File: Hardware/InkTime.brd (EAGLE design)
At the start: 36 x 36 mm, 50 parts, among them IC1 BQ25180YBGR, IC2 DRV2605YZFR, IC3 BMA423, IC9 RT6160AWSC, J1 EPD_24P, J2 TC2030, J4 USB-C, U1 nRF52840, U3 MAX17048G+T10, X1 32MHz, X2 32.768kHz

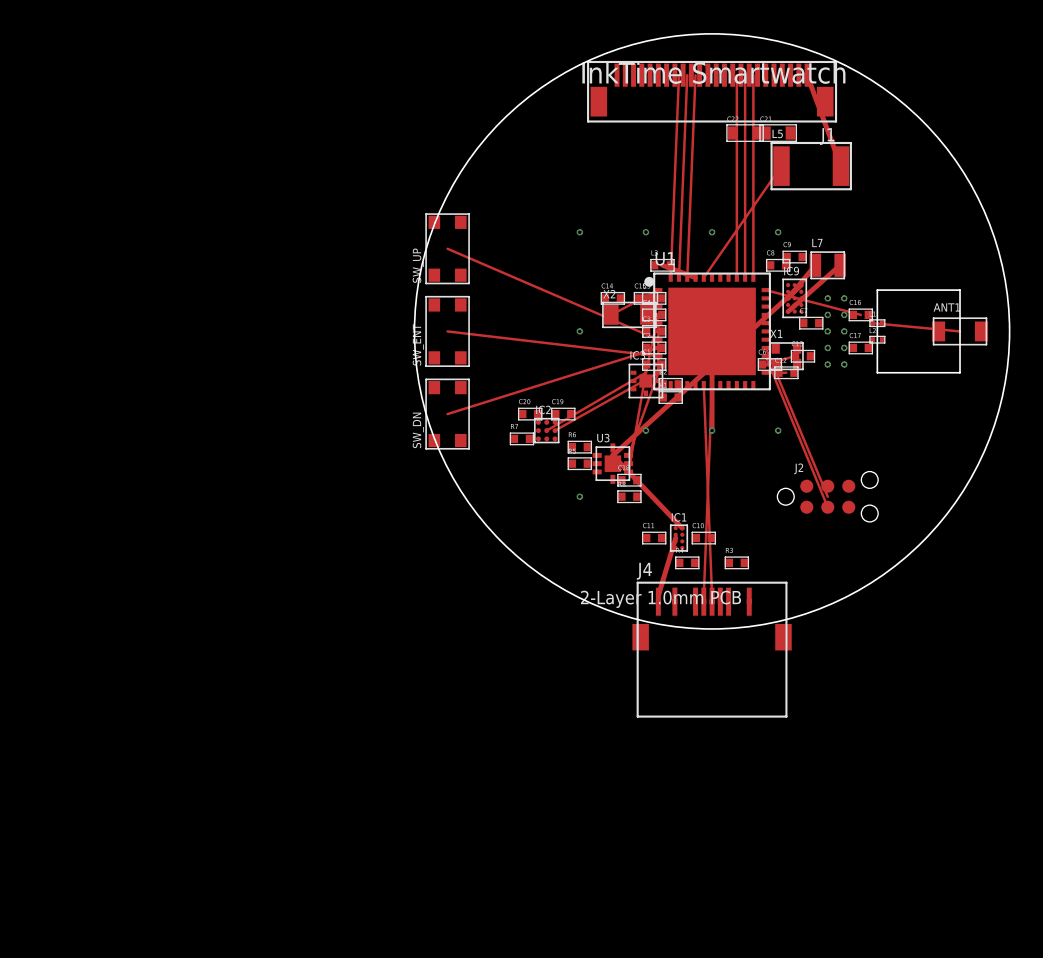
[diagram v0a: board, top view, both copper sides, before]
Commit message: Update 1
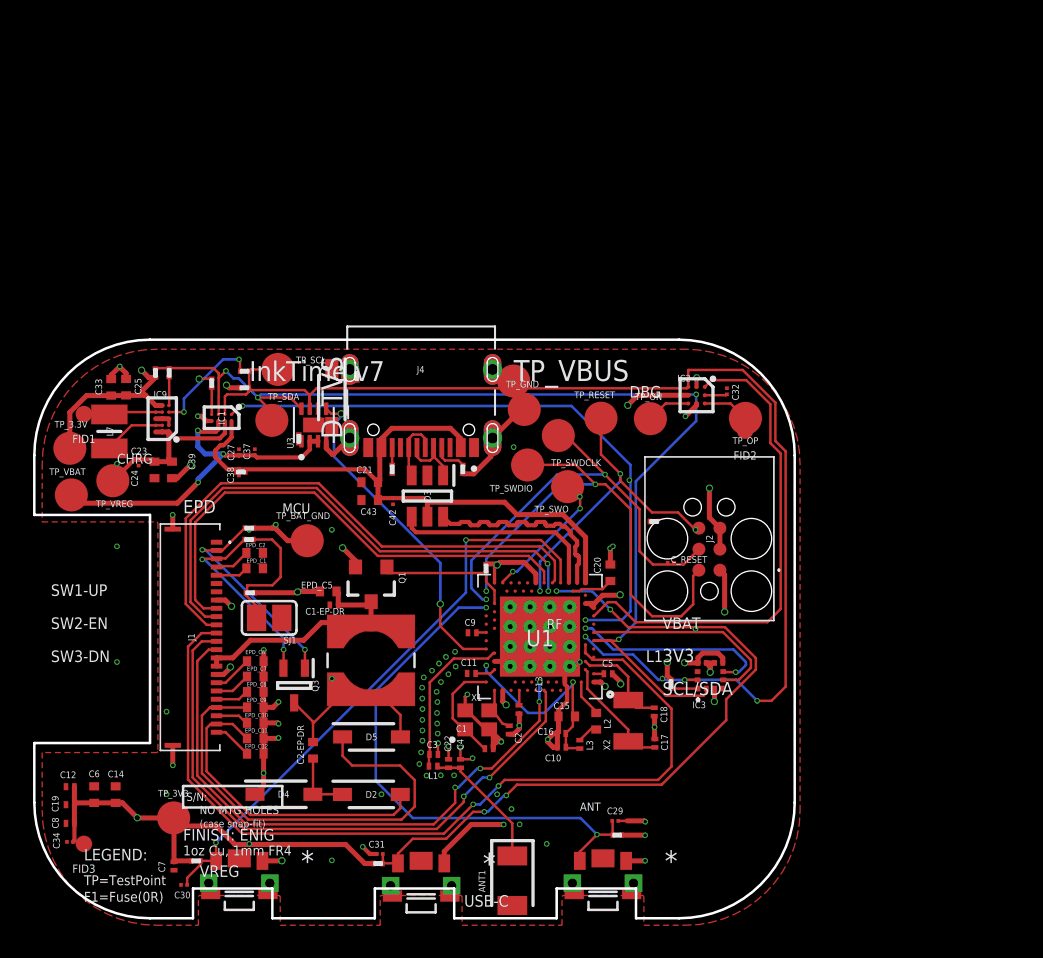
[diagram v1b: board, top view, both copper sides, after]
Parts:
- removed R1: 10k, InkTime_v5:GENERIC_0402
- removed R6: 100k, InkTime_v5:GENERIC_0402
- added C1-EP-DR, C24, C39: 10uF, InkTime_v5:NORDIC_NRF_3_RESC0402_L
- added C2-EP-DR: 4.7uF/25V, InkTime_v5:NORDIC_NRF_3_RESC0402_L
- added C23, C27, C34, C42: 0.1uF, InkTime_v5:GRM011R60J152KE01L_2_CAPC0201X13N
- added C25, C33: 22uF, InkTime_v5:NORDIC_NRF_3_RESC0402_L
- added C29, C30, C31, C32, C37, C38: 1uF, InkTime_v5:GRM011R60J152KE01L_2_CAPC0201X13N
- added C43: 4.7uF, InkTime_v5:NORDIC_NRF_3_RESC0402_L
- added C_RESET: 100nF/10V, InkTime_v5:GRM011R60J152KE01L_2_CAPC0201X13N
- added D2, D4, D5: MBR0530, InkTime_v5:ESP32_C6_LIBRARY_5_SOD3716X135N
- added D3: USBLC6-2SC6Y, InkTime_v5:ESP32_C6_LIBRARY_3_SOT95P280X145-6N
- added D_TVS: MBR0530 (TVS), InkTime_v5:ESP32_C6_LIBRARY_5_SOD3716X135N
- added EPD_C1, EPD_C10, EPD_C11, EPD_C12, EPD_C2, EPD_C6, EPD_C7, EPD_C8, EPD_C9: 1uF/50V, InkTime_v5:NORDIC_NRF_3_RESC0402_L
- added EPD_C5: 0.1uF/50V, InkTime_v5:NORDIC_NRF_3_RESC0201_L
- added F1: 0R (FUSE), InkTime_v5:CPF0201D7K68C1_0201
- added Q1: 20V/4.2A/52mΩ/1.4W, InkTime_v5:ESP32_C6_LIBRARY_4_ESP32_C6_LIBRARY_4_ESP32_C6_LIBRARY_4_ESP32_C6_LIBRARY_4_ESP32_WROVER_SPARKFUN-DISCRETESE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
- added Q3: SI1308EDL-T1-GE3, InkTime_v5:ESP32_C6_LIBRARY_6_SOT65P210X110-3N
- added R17, R18: 3K3, InkTime_v5:CPF0201D7K68C1_0201
- added R1_EP_DR: 0.47, InkTime_v5:CPF0201D7K68C1_0201
- added R1_USB, R2_USB: 5K1, InkTime_v5:CPF0201D7K68C1_0201
- added R2_EP_DR, R9, R_PWR_EPD, R_RESET: 10K, InkTime_v5:CPF0201D7K68C1_0201
- added R_ALERT, R_PMIC_INT: 100K, InkTime_v5:CPF0201D7K68C1_0201
- added R_TYPE_SEL: 2.2, InkTime_v5:CPF0201D7K68C1_0201
- added SJ1: SJ, InkTime_v5:ESP32_C6_LIBRARY_7_JUMPER_SJ
- added TP_3.3V, TP_3V3, TP_BAT_GND, TP_GND, TP_ON, TP_OP, TP_RESET, TP_SCL, TP_SDA, TP_SWDCLK, TP_SWDIO, TP_SWO, TP_VBAT, TP_VREG: HECTOR_WATCH_1_TPTP20R, InkTime_v5:HECTOR_WATCH_1_TP20R
- added TP_VBUS: VBUS, InkTime_v5:HECTOR_WATCH_1_TP20R
- ANT1: value 2450AT18B100E -> 2450AT18B100E_2450AT18B100E
- C1, C2: value 100nF -> 12pF; device InkTime_v5:GENERIC_0402 -> InkTime_v5:NORDIC_NRF_3_RESC0201_L
- C10: value 1uF -> N.C.; device InkTime_v5:GENERIC_0402 -> InkTime_v5:NORDIC_NRF_3_RESC0201_L
- C11: value 4.7uF -> 100pF; device InkTime_v5:GENERIC_0402 -> InkTime_v5:NORDIC_NRF_3_RESC0201_L
- C12: value 12pF -> 100nF; device InkTime_v5:GENERIC_0402 -> InkTime_v5:NORDIC_NRF_3_RESC0201_L
- C13: value 12pF -> N.C.; device InkTime_v5:GENERIC_0402 -> InkTime_v5:NORDIC_NRF_3_RESC0201_L
- C14: value 6.8pF -> 4.7uF; device InkTime_v5:GENERIC_0402 -> InkTime_v5:NORDIC_NRF_3_RESC0402_L
- C15: value 6.8pF -> 1uF; device InkTime_v5:GENERIC_0402 -> InkTime_v5:NORDIC_NRF_3_RESC0402_L
- C16: value 0.8pF -> 47nF; device InkTime_v5:GENERIC_0402 -> InkTime_v5:NORDIC_NRF_3_RESC0201_L
- C17: value 0.5pF -> 12pF; device InkTime_v5:GENERIC_0402 -> InkTime_v5:NORDIC_NRF_3_RESC0201_L
- C18: value 1uF -> 12pF; device InkTime_v5:GENERIC_0402 -> InkTime_v5:NORDIC_NRF_3_RESC0201_L
- C19: value 1uF -> 100nF; device InkTime_v5:GENERIC_0402 -> InkTime_v5:NORDIC_NRF_3_RESC0201_L
- C20: value 100nF -> 4.7uF; device InkTime_v5:GENERIC_0402 -> InkTime_v5:NORDIC_NRF_3_RESC0402_L
- C21: device InkTime_v5:GENERIC_0603 -> InkTime_v5:NORDIC_NRF_3_RESC0402_L
- C22: value 1uF -> N.C.; device InkTime_v5:GENERIC_0603 -> InkTime_v5:NORDIC_NRF_3_RESC0201_L
- C3: value 100nF -> 1pF; device InkTime_v5:GENERIC_0402 -> InkTime_v5:NORDIC_NRF_3_RESC0201_L
- C4: value 1uF -> 1pF; device InkTime_v5:GENERIC_0402 -> InkTime_v5:NORDIC_NRF_3_RESC0201_L
- C5: device InkTime_v5:GENERIC_0402 -> InkTime_v5:NORDIC_NRF_3_RESC0201_L
- C6: device InkTime_v5:GENERIC_0402 -> InkTime_v5:NORDIC_NRF_3_RESC0402_L
- C7, C8: value 10uF -> 100nF; device InkTime_v5:GENERIC_0402 -> InkTime_v5:NORDIC_NRF_3_RESC0201_L
- C9: value 100nF -> 820pF (N.C.); device InkTime_v5:GENERIC_0402 -> InkTime_v5:NORDIC_NRF_3_RESC0201_L
- IC1: value BQ25180YBGR -> BQ25180YBGR_BQ25180YBGR
- IC2: value DRV2605YZFR -> DRV2605YZFR_DRV2605YZFR
- IC3: value BMA423 -> BMA423_BMA423
- IC9: value RT6160AWSC -> RT6160AWSC_RT6160AWSC
- J1: value EPD_24P -> 503480-2400_503480-2400
- J2: value TC2030 -> TC2030-IDC_TC2030-IDC
- J4: value USB-C -> KH-TYPE-C-16P
- L2: value 15nH -> 10uH; device InkTime_v5:NORDIC_NRF_2_RESC0201_L -> InkTime_v5:NORDIC_NRF_2_RESC0402_L
- L3: value 10uH -> 15nH; device InkTime_v5:NORDIC_NRF_2_RESC0402_L -> InkTime_v5:NORDIC_NRF_2_RESC0201_L
- L7: value 4.7uH -> MLP2016SR47MT0S1_FTC252012SR47MBCA
- R2: value 10k -> 0; device InkTime_v5:GENERIC_0402 -> InkTime_v5:CPF0201D7K68C1_0201
- R3, R4: value 5.1k -> 0; device InkTime_v5:GENERIC_0402 -> InkTime_v5:CPF0201D7K68C1_0201
- R5: value 100k -> 10K; device InkTime_v5:GENERIC_0402 -> InkTime_v5:CPF0201D7K68C1_0201
- R7: value 4.7k -> 10K; device InkTime_v5:GENERIC_0402 -> InkTime_v5:CPF0201D7K68C1_0201
- R8: value 1M -> 10K; device InkTime_v5:GENERIC_0402 -> InkTime_v5:CPF0201D7K68C1_0201
- SW_DN: value SW_DN -> 2025-10-22_07-23-44_LIBRARY_EVP-AKE31ASW_EVP-AKE31A_PAN
- SW_ENT: value SW_ENT -> 2025-10-22_07-23-44_LIBRARY_EVP-AKE31ASW_EVP-AKE31A_PAN
- SW_UP: value SW_UP -> 2025-10-22_07-23-44_LIBRARY_EVP-AKE31ASW_EVP-AKE31A_PAN
- U1: value nRF52840 -> NORDIC_NRF_4_NRF52840_QF
- moved C8 54.5 mm to (-20.8, -11.8), turned to 180 degrees
- moved C7 50.6 mm to (-14.6, -14.3), turned to 270 degrees
- moved C12 50.0 mm to (-20.8, -9.54), turned to 180 degrees
- moved C6 48.5 mm to (-19.4, -10.0), turned to 90 degrees
- moved J1 46.3 mm to (-13.5, -0.50), turned to 270 degrees
- moved L7 44.6 mm to (-18.5, 11.9), turned to 90 degrees
- moved ANT1 42.9 mm to (5.92, -15.2), turned to 270 degrees
- moved C14 42.5 mm to (-18.1, -10.0), turned to 90 degrees
- moved C22 42.1 mm to (2.06, -8.14), turned to 90 degrees
- moved L5 40.0 mm to (-2.63, -1.90), turned to 90 degrees
- moved SW_UP 40.0 mm to (-10.6, -15.0), turned to 180 degrees
- moved IC9 38.9 mm to (-15.3, 12.7), turned to 180 degrees
- moved C19 38.1 mm to (-20.8, -10.6), turned to 180 degrees
- moved L1 38.0 mm to (1.13, -8.30)
- moved R5 33.4 mm to (-13.2, -14.0), turned to 270 degrees
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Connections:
- removed net ACC_INT1: IC3.5, U1.10
- removed net ANT: C16.1, L1.1, U1.33
- removed net ANT_GND: C17.2, L2.2
- removed net ANT_MATCH: ANT1.2, C16.2, C17.1, L1.2, L2.1
- removed net BTN_DN: SW_DN.1, U1.8
- removed net BTN_ENT: SW_ENT.1, U1.9
- removed net BTN_UP: SW_UP.1, U1.7
- removed net CC1: J4.A5, R3.2
- removed net CC2: J4.B5, R4.2
- removed net CHG_STAT: IC1.B1, U1.12
- removed net DEC1: L3.1, U1.30
- removed net DEC4: U1.29
- removed net EPD_MOSI: J1.8, U1.35
- removed net EPD_SCK: J1.7, U1.34
- removed net EPD_VDD: C21.1, C22.1, J1.1, L5.2
- removed net EPD_VSW: L5.1, U1.40
- removed net FUEL_ALRT: U1.11, U3.3
- removed net HAPTIC_OUT: IC2.A1
- removed net NFC1: U1.14
- removed net NFC2: U1.13
- removed net SCL_PU: R2.2
- removed net SDA_PU: R1.2
- removed net SW: IC9.C1, L7.1
- removed net SWD_RST: J2.5, U1.22
- removed net USB_DN: J4.A7, U1.16
- removed net USB_DP: J4.A6, U1.17
- removed net VDD: C1.1, C2.1, C3.1, C4.1, C5.1, C6.1, IC9.A1, L3.2, U1.37, U1.38, U1.39
- removed net VSYS: C8.1, IC9.E1, L7.2
- removed net XC1: C12.1, U1.23, X1.1
- removed net XC2: C13.1, U1.24, X1.2
- removed net XL1: C14.1, U1.1, X2.1
- removed net XL2: C15.1, U1.2, X2.2
- new net 3V3: C12.1, C14.1, C19.1, C25.1, C33.1, C34.1, C6.1, C7.1, C8.1, IC2.C2, IC3.10, IC3.3, IC3.7, IC9.E2, IC9.E3, J2.1, Q1.2, R17.1, R18.1, R5.2, R7.2, R8.2, R_ALERT.2, R_PMIC_INT.2, R_PWR_EPD.2, R_RESET.2, TP_3.3V.TP, TP_3V3.TP, U1.P$A22, U1.P$AD14, U1.P$AD23, U1.P$B1, U1.P$W1, U1.P$Y2
- new net ALERT: R_ALERT.1, U1.P$J24, U3.5
- new net D+: D3.4, U1.P$AD6
- new net D-: D3.6, U1.P$AD4
- new net DEC4_6: C10.1, C15.1, C16.1, L3.2, U1.P$B5, U1.P$E24
- new net DN: D3.1, J4.A7, J4.B7
- new net DP: D3.3, J4.A6, J4.B6
- new net EPD_3V3: C1-EP-DR.1, EPD_C5.2, J1.15, J1.16, L5.2, Q1.3
- new net GDR: J1.2, Q3.1, R2_EP_DR.2
- new net HAPTIC_EN: IC2.A1, U1.P$U1
- new net IMU_INT1: IC3.5, U1.P$N1
- new net IMU_INT2: IC3.6, U1.P$P2
- new net LX1: IC9.B2, IC9.B3, L7.1
- new net LX2: IC9.D2, IC9.D3, L7.2
- new net MOSI: J1.14, U1.P$B13
- new net N$1: L2.2, L3.1
- new net N$10: EPD_C6.2, J1.18
- new net N$11: R1_EP_DR.1, R_TYPE_SEL.2, SJ1.2
- new net N$12: J4.A5, R1_USB.2
- new net N$14: EPD_C2.2, J1.4
- new net N$15: EPD_C1.2, J1.5
- new net N$16: J4.B5, R2_USB.1
- new net N$18: EPD_C7.2, J1.19
- new net N$19: C2-EP-DR.2, D5.2, L5.1, Q3.3
- new net N$2: IC9.D1, R4.1
- new net N$20: C20.1, U1.P$AC5
- new net N$21: EPD_C8.2, J1.20
- new net N$22: EPD_C12.2, J1.24
- new net N$24: EPD_C10.2, J1.22
- new net N$3: C32.1, IC2.A2
- new net N$4: IC9.E1, R2.1
- new net N$40: L2.1, U1.P$B3
- new net N$43: C13.1, U1.P$A18
- new net N$58: C9.1, U1.P$N24
- new net N$59: C11.1, U1.P$D23
- new net N$6: IC3.1, R3.1
- new net N$60: C2.1, U1.P$A23, X1.3
- new net N$61: C1.1, U1.P$B24, X1.1
- new net N$62: C3.1, L1.1, U1.P$H23
- new net N$63: ANT1.1, C22.1, C4.1, L1.2
- new net N$7: C5.1, U1.P$C1
- new net N$8: IC1.D1, R9.2
- new net N$9: C2-EP-DR.1, D2.1, D4.2
- new net OUT+: IC2.A3, TP_OP.TP
- new net OUT-: IC2.C3, TP_ON.TP
- new net P0.00/XL1: C17.2, U1.P$D2, X2.2
- new net P0.00/XL2: C18.2, U1.P$F2, X2.1
- new net P0.04: U1.P$J1
- new net P0.09: U1.P$L24
- new net P0.13: C30.1, R5.1, SW_UP.2, U1.P$AD8
- new net P0.14: C31.1, R8.1, SW_ENT.2, U1.P$AC9
- new net P0.19: U1.P$AC15
- new net P0.20: U1.P$AD16
- new net P0.21: U1.P$AC17
- new net P0.22: U1.P$AD18
- new net P0.23: U1.P$AC19
- new net P0.24: U1.P$AD20
- new net P0.25: U1.P$AC21
- new net P0.26: U1.P$G1
- new net P0.27: U1.P$H2
- new net P0.28: U1.P$B11
- new net P0.29: U1.P$A10
- new net P0.30: U1.P$B9
- new net P0.31: U1.P$A8
- new net P1.01: Q1.1, R_PWR_EPD.1, U1.P$Y23
- new net P1.02: C29.1, R7.1, SW_DN.2, U1.P$W24
- new net P1.03: U1.P$V23
- new net P1.04: U1.P$U24
- new net P1.05: U1.P$T23
- new net P1.06: U1.P$R24
- new net P1.07: U1.P$P23
- new net P1.09: U1.P$R1
- new net P1.10: U1.P$A20
- new net P1.11: U1.P$B19
- new net P1.12: U1.P$B17
- new net P1.13: U1.P$A16
- new net P1.14: U1.P$B15
- new net P1.15: U1.P$A14
- new net PMIC_INT: IC1.A1, R_PMIC_INT.1, U1.P$T2
- new net PREVGH: D5.1, EPD_C9.2, J1.21
- new net PREVGL: D2.2, EPD_C11.2, J1.23
- new net RESE: J1.3, Q3.2, R1_EP_DR.2
- new net RESET: C_RESET.1, J2.6, R_RESET.1, TP_RESET.TP, U1.P$AC13
- new net SCK: J1.13, U1.P$A12
- new net SWO: TP_SWO.TP, U1.P$AD22
- new net VREG: C23.1, C24.2, C39.1, IC1.B2, IC9.A1, IC9.A2, IC9.A3, TP_VREG.TP
- net EPD_BUSY: now also J1.9, U1.P$AD12; no longer J1.12, U1.44
- net EPD_CS: now also J1.12, U1.P$K2; no longer J1.9, U1.36
- net EPD_DC: now also J1.11, U1.P$AD10; no longer J1.10, U1.42
- net EPD_RST: now also J1.10, U1.P$AC11; no longer J1.11, U1.43
- net GND: now also C1-EP-DR.2, C16.2, C17.1, C18.1, C23.2, C24.1, C25.2, C27.2, C29.2, C30.2, C31.2, C32.2, C33.2, C34.2, C37.2, C38.2, C39.2, C42.2, C43.2, C_RESET.2, D3.2, D4.1, D_TVS.1, EPD_C1.1, EPD_C10.1, EPD_C11.1, EPD_C12.1, EPD_C2.1, EPD_C5.1, EPD_C6.1, EPD_C7.1, EPD_C8.1, EPD_C9.1, IC2.B1, IC2.B3, IC3.8, IC3.9, IC9.B1, IC9.C1, IC9.C2, IC9.C3, J1.17, J1.8, J1.MP1, J1.MP2, J2.3, J2.5, J4.A12_B1, J4.A1_B12, J4.SH1, J4.SH2, J4.SH3, J4.SH4, R1_USB.1, R2_EP_DR.1, R2_USB.2, R3.2, R9.1, R_TYPE_SEL.1, SJ1.1, SW_DN.1, SW_ENT.1, SW_UP.1, TP_BAT_GND.TP, TP_GND.TP, U1.P$74, U1.P$75, U1.P$76, U1.P$77, U1.P$78, U1.P$79, U1.P$80, U1.P$81, U1.P$82, U1.P$83, U1.P$84, U1.P$85, U1.P$86, U1.P$87, U1.P$88, U1.P$89, U1.P$90, U1.P$B7, U1.P$F23, U3.1, U3.4, U3.6, U3.9, X1.2; no longer ANT1.1, C18.2, IC2.C2, IC3.GND, IC9.E2, J1.S1, J1.S2, J4.S1, J4.S2, SW_DN.2, SW_DN.4, SW_ENT.2, SW_ENT.4, SW_UP.2, SW_UP.4, U1.GND, U3.GND, X1.3
- net SCL: now also IC1.B1, IC2.C1, IC3.12, R17.2, R4.2, TP_SCL.TP, U1.P$M2; no longer IC2.B3, IC3.7, R2.1, U1.5
- net SDA: now also IC1.C1, IC2.B2, IC3.2, R18.2, R2.2, TP_SDA.TP, U1.P$L1, U3.8; no longer IC2.B1, IC3.1, R1.1, U1.4, U3.5
- net SWDCLK: now also TP_SWDCLK.TP, U1.P$AA24; no longer U1.25
- net SWDIO: now also TP_SWDIO.TP, U1.P$AC24; no longer U1.26
- net VBAT: now also C27.1, C37.1, IC1.C2, TP_VBAT.TP, U3.2, U3.3; no longer C11.1, IC1.A2, IC9.A3, U3.1
- net VBUS: now also C21.1, C38.1, C42.1, C43.1, D3.5, D_TVS.2, F1.1, F1.2, IC1.A2, J4.A4_B9, J4.A9_B4, TP_VBUS.TP, U1.P$AD2; no longer IC1.A1, J4.A1, J4.B1, R3.1, R4.1
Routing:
- net GND: track 6.00 -> 97.5 mm, vias 19 -> 84
- net 3V3: track 0.00 -> 61.6 mm, vias 0 -> 13
- net SCL: track 15.5 -> 73.7 mm, vias 0 -> 3
- net SDA: track 16.6 -> 67.8 mm, vias 0 -> 4
- net P0.14: track 0.00 -> 43.5 mm, vias 0 -> 4
- net EPD_CS: track 12.2 -> 53.0 mm, vias 0 -> 2
- net PMIC_INT: track 0.00 -> 37.6 mm, vias 0 -> 2
- net VBUS: track 3.65 -> 40.9 mm
- net SCK: track 0.00 -> 36.8 mm, vias 0 -> 2
- net P0.13: track 0.00 -> 36.0 mm, vias 0 -> 2
- net MOSI: track 0.00 -> 35.8 mm, vias 0 -> 4
- net P1.02: track 0.00 -> 32.8 mm, vias 0 -> 2
- net HAPTIC_EN: track 0.00 -> 29.9 mm
- net PREVGH: track 0.00 -> 28.5 mm
- net EPD_DC: track 12.3 -> 34.1 mm
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- added copper zone on layer 15, net 3V3
- added copper zone on layer 1, net GND
- added copper zone on layer 2, net GND
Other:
- board size 36 x 36 mm -> 46 x 35 mm
- board text added: "(case snap-fit)"
- board text added: "1oz Cu, 1mm FR4"
- board text added: "3V3"
- board text added: "ANT"
- board text added: "CHRG"
- board text added: "DBG"
- board text added: "EPD"
- board text added: "F1=Fuse(0R)"
- board text added: "FID1"
- board text added: "FID2"
- board text added: "FID3"
- board text added: "FINISH: ENIG"
- board text added: "GND pour"
- board text added: "InkTime v7"
- board text added: "L1"
- board text added: "L2"
- board text added: "LEGEND:"
- board text added: "MCU"
- board text added: "NO MTG HOLES"
- board text added: "RF"
- board text added: "S/N:"
- board text added: "SCL/SDA"
- board text added: "SW1-UP"
- board text added: "SW2-EN"
- board text added: "SW3-DN"
- board text added: "TP=TestPoint"
- board text added: "USB-C"
- board text added: "VBAT"
- board text added: "VREG"
- board text added: "bot.GND"
- board text removed: "2-Layer 1.0mm PCB"
- board text removed: "InkTime Smartwatch"
